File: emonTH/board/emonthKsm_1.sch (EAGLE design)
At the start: 9 parts

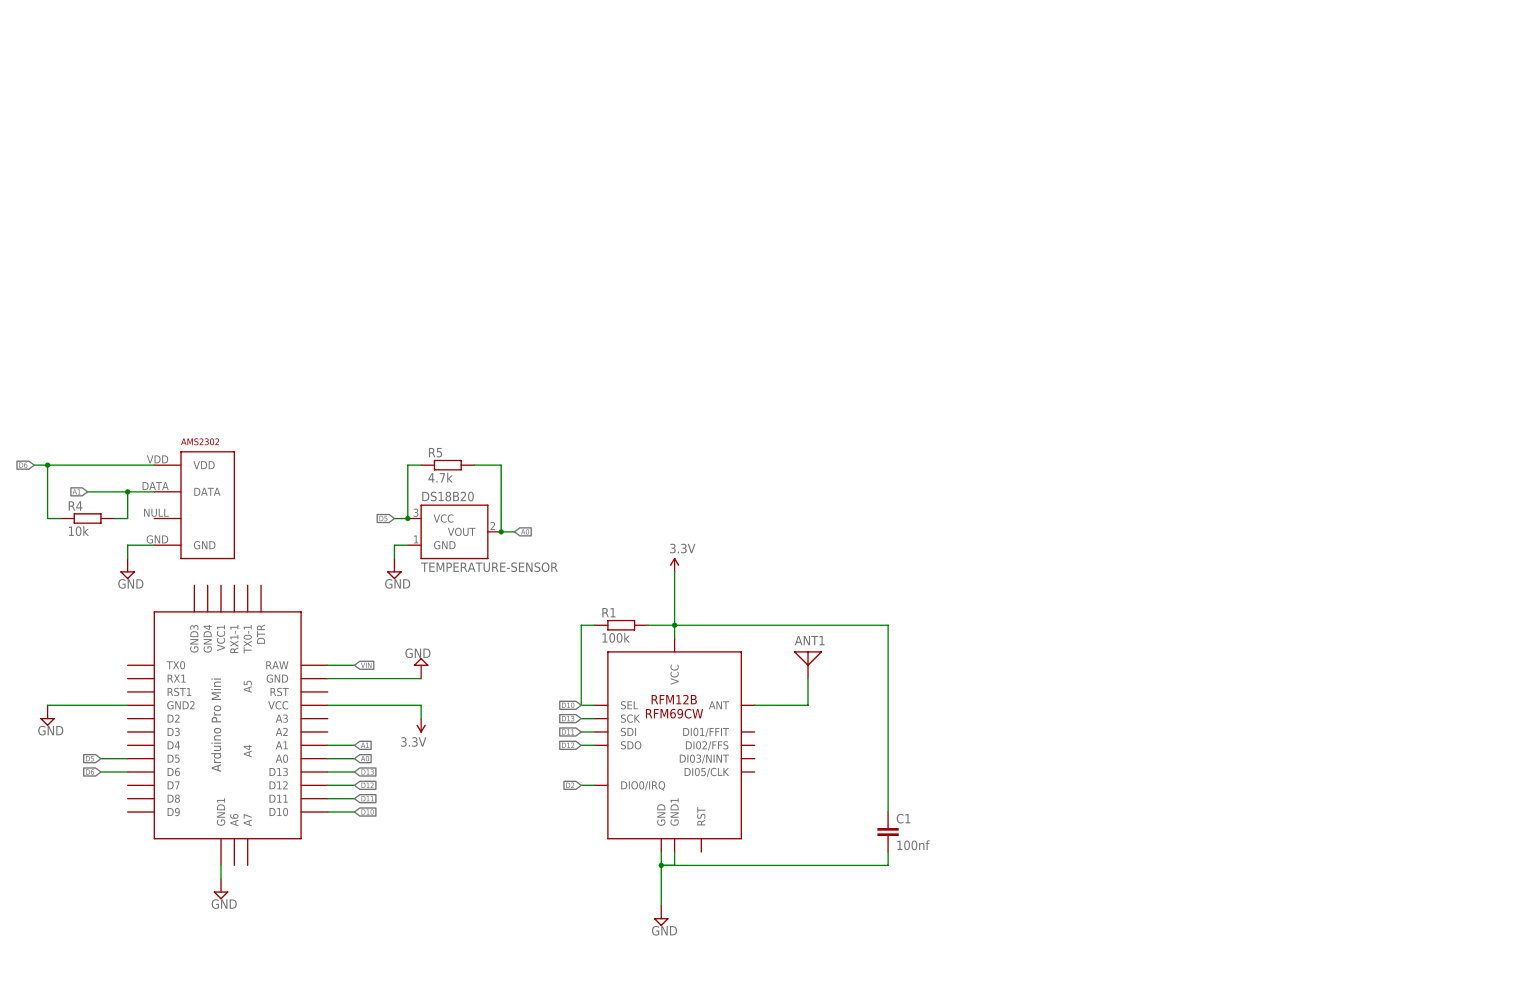
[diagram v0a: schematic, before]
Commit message: Update emonthKSM board
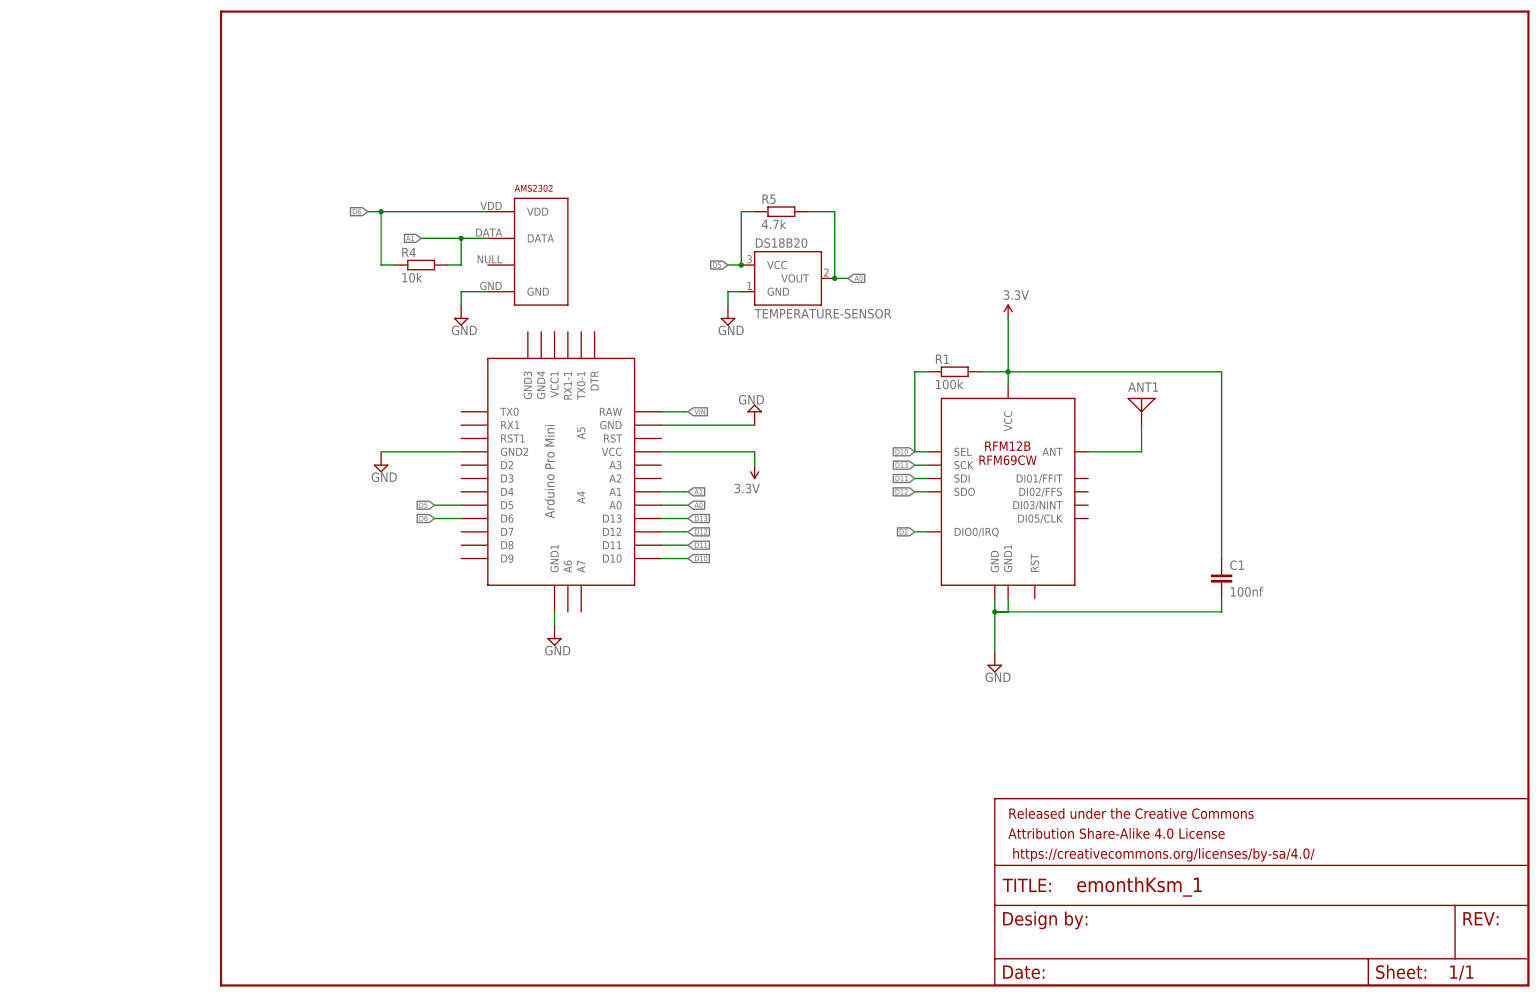
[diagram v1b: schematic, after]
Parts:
- added FRAME1: FRAME-LETTERNO_PACKAGE, SparkFun-Aesthetics:FRAME-LETTERNO_PACKAGE
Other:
- moved on the sheet: AMS2302, ANT1, C1, DS18B20, R1, R4, R5
